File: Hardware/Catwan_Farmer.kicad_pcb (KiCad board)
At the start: 2 copper layers, 60 x 70 mm, 56 parts, among them J1 SENSOR 1, J10 VSP, J2 SENSOR 2, J3 SENSOR 3, J4 BATT, J5 USB_B, J6 Conn_01x04, J7 DHT22, J9 SENSOR 4, SW1 SW_Push, U1 AP2114N-1.0, U2 RFM95W-915S2, U3 ATSAMD21E18A-MU, U4 MCP73831-4-OT, U5 74HC4052, Y1 32.768Khz

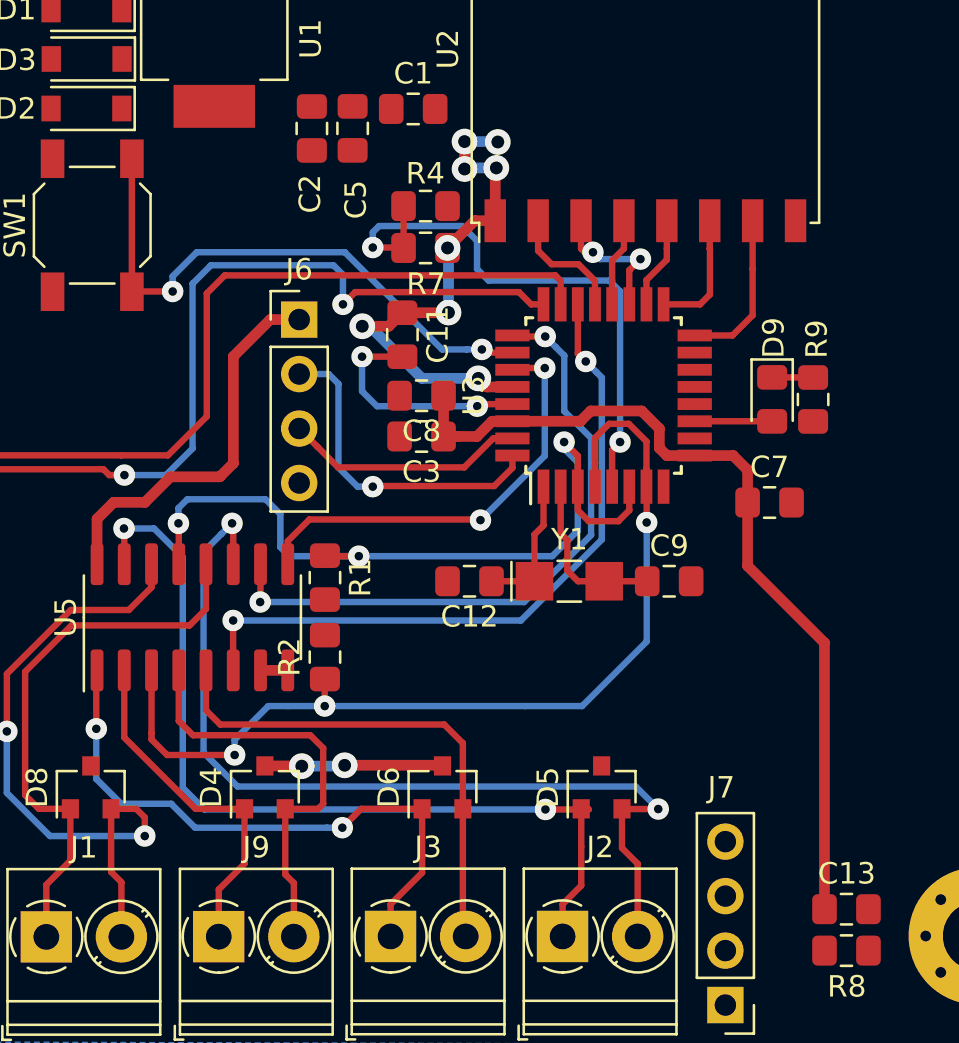
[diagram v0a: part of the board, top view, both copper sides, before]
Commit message: delete tracks
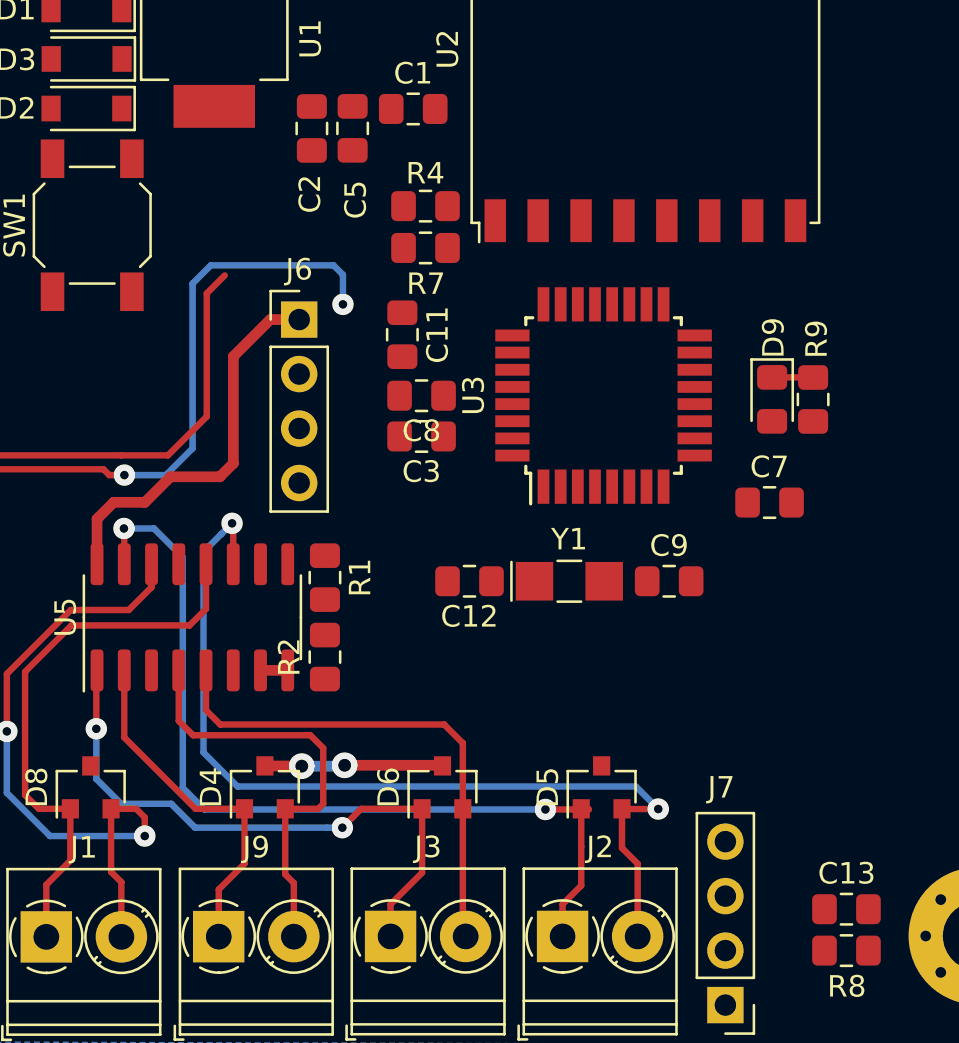
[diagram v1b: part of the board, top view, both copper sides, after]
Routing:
- net /SENS_Y: track 45.9 -> 0.00 mm, vias 3 -> 0
- net +3V3: track 58.5 -> 18.3 mm
- net /SENS_X: track 37.3 -> 0.00 mm, vias 3 -> 0
- net /EN: track 32.5 -> 0.00 mm, vias 2 -> 0
- net /S0: track 30.2 -> 0.00 mm, vias 2 -> 0
- net Net-(SW1-Pad2): track 27.1 -> 0.00 mm, vias 2 -> 0
- net /ADC_BAT: track 27.0 -> 0.00 mm, vias 2 -> 0
- net GND: track 34.6 -> 9.58 mm, vias 10 -> 2
- net /S1: track 20.4 -> 0.00 mm, vias 2 -> 0
- net /D-: track 37.3 -> 20.4 mm
- net /SWDIO: track 15.3 -> 0.00 mm, vias 1 -> 0
- net /SWCLK: track 11.2 -> 0.00 mm
- net Net-(C11-Pad2): track 10.8 -> 0.00 mm, vias 2 -> 0
- net /D+: track 39.1 -> 29.3 mm
- net /Y1: track 7.97 -> 0.00 mm
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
